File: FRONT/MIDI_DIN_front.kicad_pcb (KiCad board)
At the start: 2 copper layers, 30 x 128.5 mm, 6 parts, among them J1 Screw_Terminal_01x01, J2 Screw_Terminal_01x01, J3 Screw_Terminal_01x01, J4 Screw_Terminal_01x01

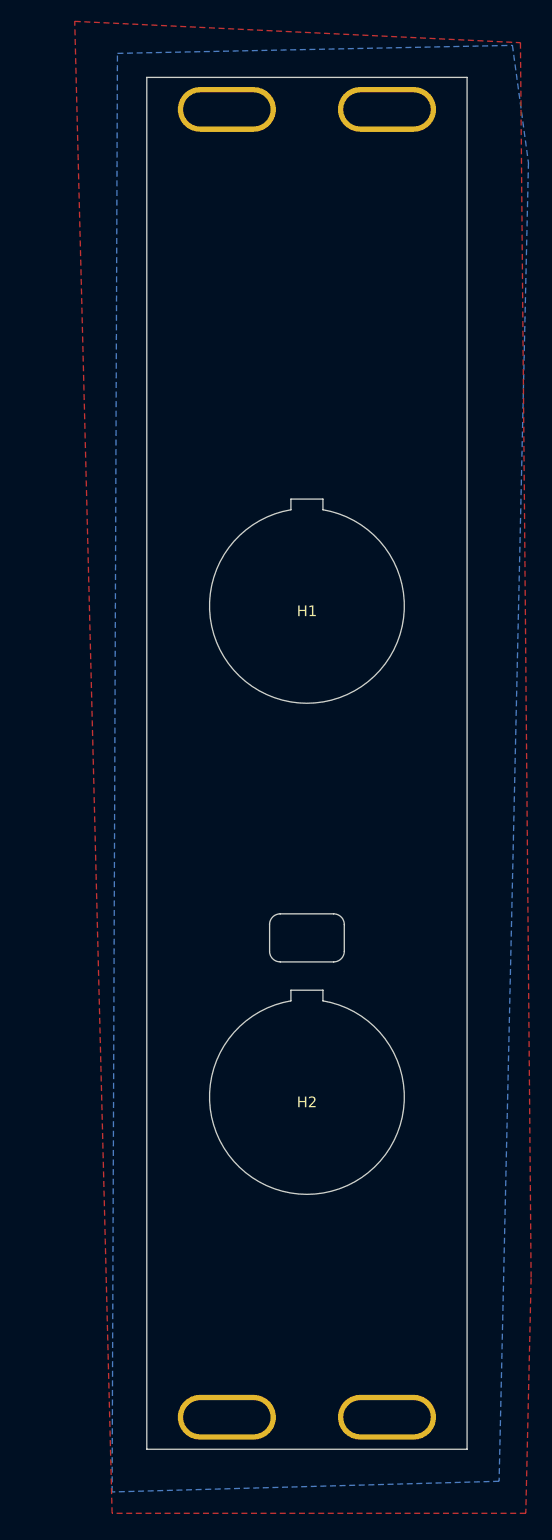
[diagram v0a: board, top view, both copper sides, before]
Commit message: Finalize module
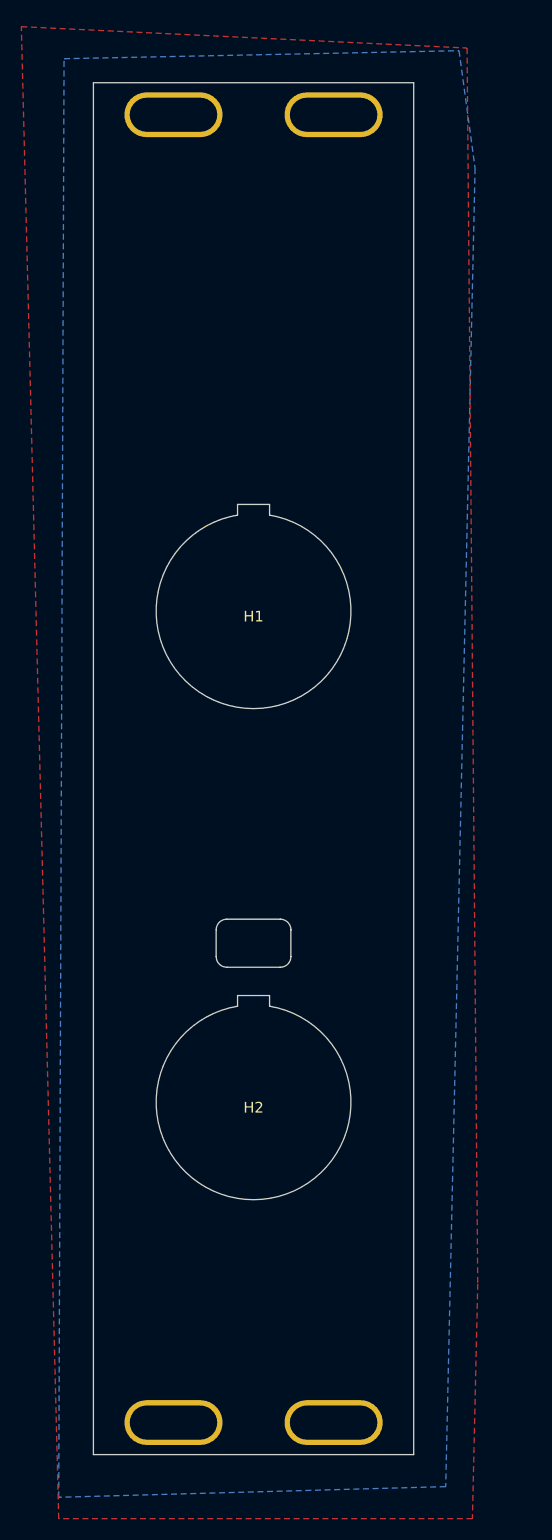
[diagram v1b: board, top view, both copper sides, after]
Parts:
- moved H1 5.02 mm to (85.0, 90.0)
- moved H2 5.02 mm to (85.0, 136.0)
- moved J1 5.02 mm to (92.5, 166.0)
- moved J2 5.02 mm to (92.5, 43.5)
- moved J3 5.02 mm to (77.5, 166.0)
- moved J4 5.02 mm to (77.5, 43.5)
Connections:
- J1 pad 1: unconnected-(J1-Pin_1-Pad1) -> Net-(J1-Pin_1)
- J2 pad 1: unconnected-(J2-Pin_1-Pad1) -> Net-(J1-Pin_1)
- J3 pad 1: unconnected-(J3-Pin_1-Pad1) -> Net-(J1-Pin_1)
- J4 pad 1: unconnected-(J4-Pin_1-Pad1) -> Net-(J1-Pin_1)
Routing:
- added copper zone on B.Cu, net Net-(J1-Pin_1)
- added copper zone on F.Cu, net Net-(J1-Pin_1)
- removed copper zone on B.Cu, net unconnected-(J2-Pin_1-Pad1)
- removed copper zone on F.Cu, net unconnected-(J2-Pin_1-Pad1)
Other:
- rule pad_to_mask_clearance: 0.05 -> 0
